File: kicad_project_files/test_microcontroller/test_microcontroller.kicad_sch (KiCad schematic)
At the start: 40 parts, among them SW1 SW_Push, SW2 SW_Push, SW3 SW_Push, SW4 SW_Push, SW5 SW_Push, SW6 SW_Push, SW7 SW_Push, SW8 SW_Push, SW9 SW_Push, U1 ATmega8U2-A, Y1 16mhz

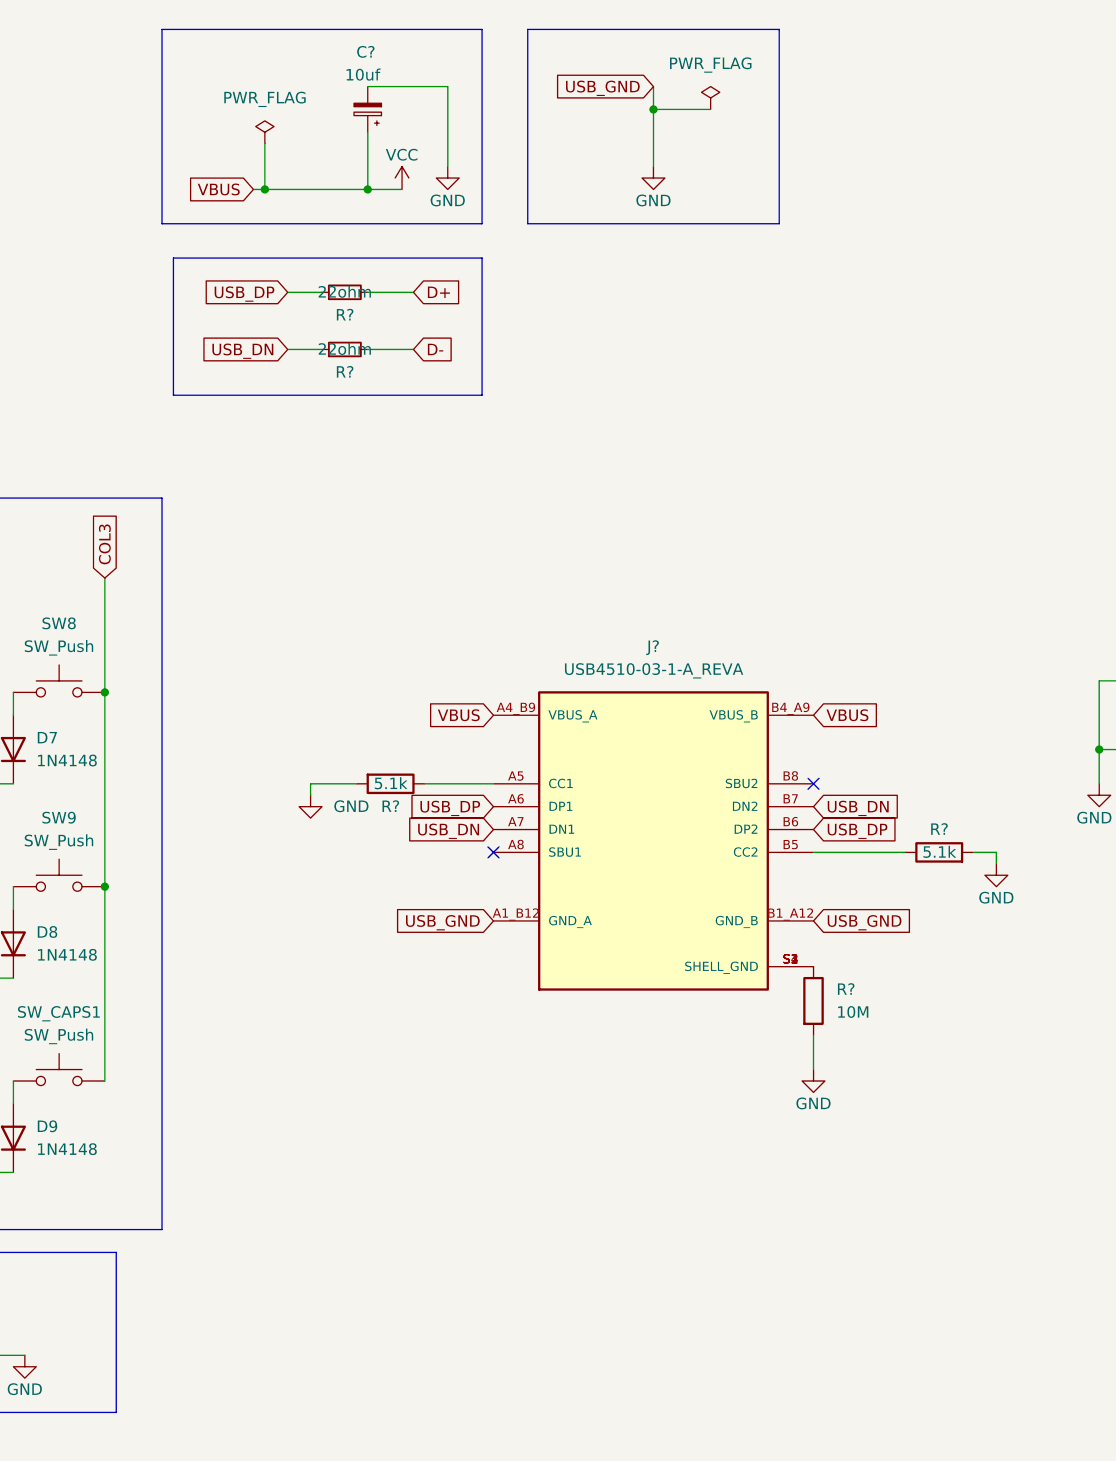
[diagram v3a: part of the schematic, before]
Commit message: update pcb - new usb
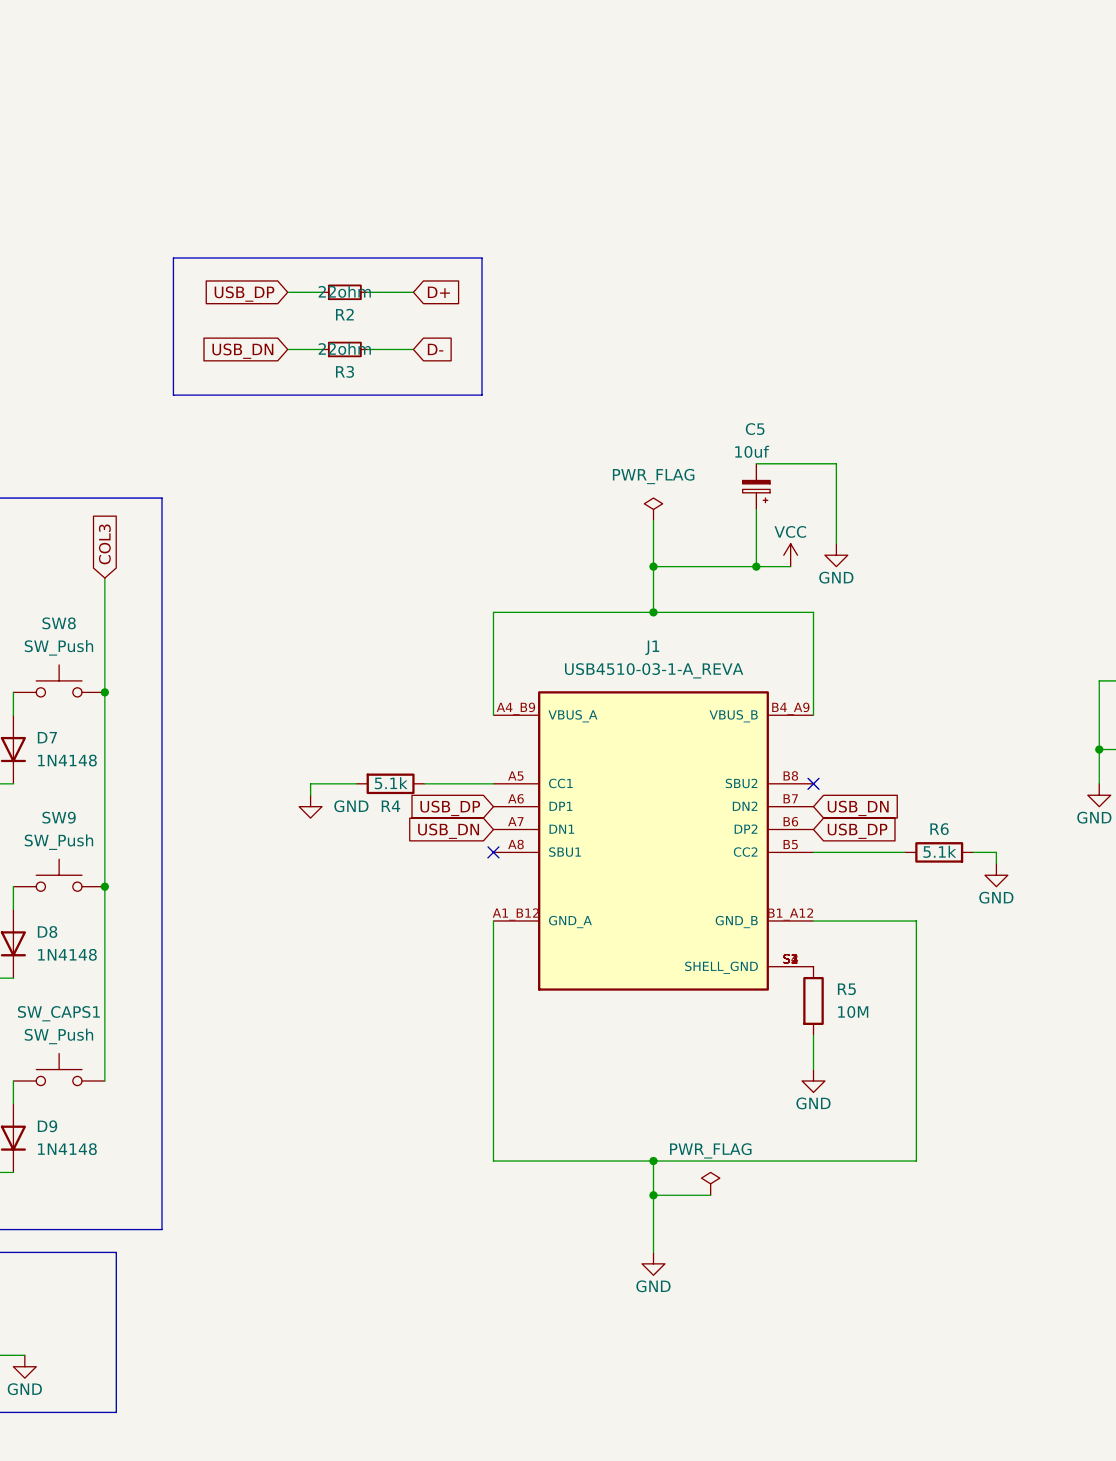
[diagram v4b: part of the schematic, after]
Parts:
- removed C?: 10uf, Capacitor_THT:CP_Radial_D4.0mm_P1.50mm, symbol Device:C_Polarized_Small
- added C5: 10uf, Capacitor_THT:CP_Radial_D4.0mm_P1.50mm, symbol Device:C_Polarized_Small
- D_CAPS1: footprint LED_SMD:LED_Cree-PLCC4_3.2x2.8mm_CCW -> CLA1A_SMD_LED:CLA1A-WKW-CXAYB153
- J1: renamed from J?; footprint GCT_USB4510-03-1-A_REVA -> GCT_USB4510-03-1-A_REVA:GCT_USB4510-03-1-A_REVA
- gave numbers to parts that had none: 5
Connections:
- net GND: now also C5.2
- net VCC: now also C5.1
